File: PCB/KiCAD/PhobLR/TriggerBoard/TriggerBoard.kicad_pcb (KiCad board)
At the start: 2 copper layers, 41.7 x 9.7 mm, 7 parts, among them J1 L, J2 R, SW1 L, SW2 R

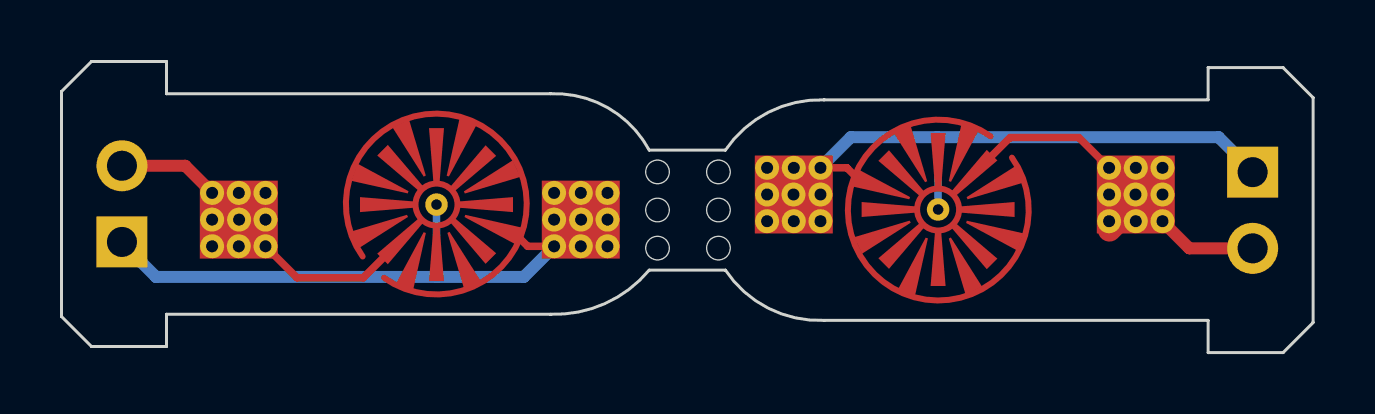
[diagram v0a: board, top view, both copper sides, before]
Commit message: .
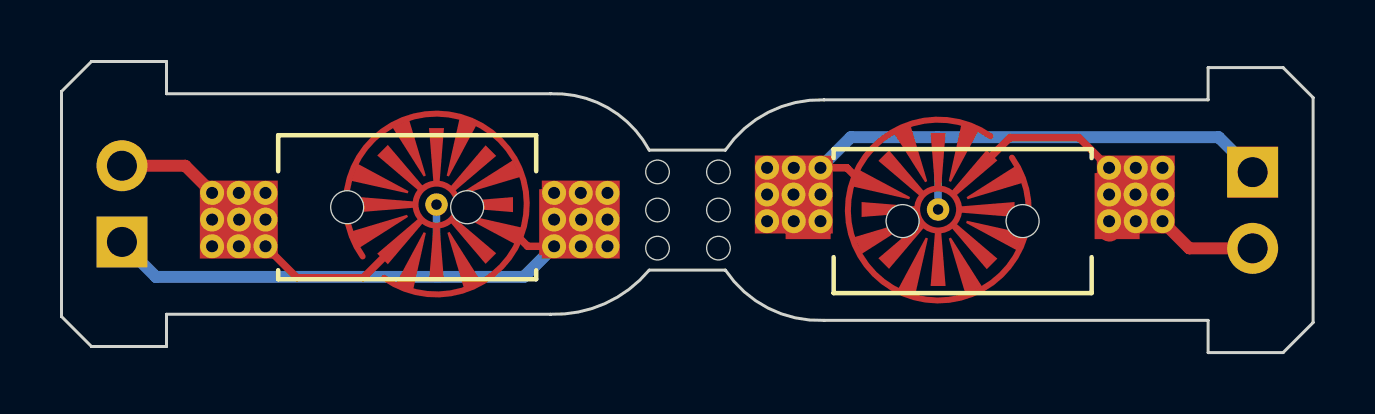
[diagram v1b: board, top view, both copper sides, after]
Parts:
- removed G*** (x2): LOGO, Library:phobtv_bold_smol
- added ?: , clipboard:b50812ef-01b3-4199-b131-0dd827ad1ccd, F.Cu at (35.7, 19.0)
- added ?: , clipboard:b50812ef-01b3-4199-b131-0dd827ad1ccd, F.Cu at (42.3, 24.5)
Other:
- board text removed: "Zinnia 2.0.5"
